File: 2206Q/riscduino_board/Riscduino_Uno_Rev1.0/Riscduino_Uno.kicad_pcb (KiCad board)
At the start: 2 copper layers, 70.1 x 54.4 mm, 93 parts, among them J1 USB_B_Micro, J10 Conn_01x01, J11 Conn_01x01, J2 ISP, J3 Conn_01x08_Pin, J4 Conn_01x06_Pin, J5 Conn_01x08_Pin, J6 Conn_01x10_Pin, J7 Conn_02x04_Odd_Even, J8 Conn_01x01, J9 Conn_01x01, SW1 4Pin Round Button SPST Straig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, U1 LM1117S-ADJ, U2 LM1117MP-3.3, U3 Riscduino, U4 CH340C, U5 MAX1232ESA+T, U6 W25Q32JVSS, U7 W25Q32JVSS, U8 23LC1024-I/P, X1 ASE-10.000MHZ-LC-T

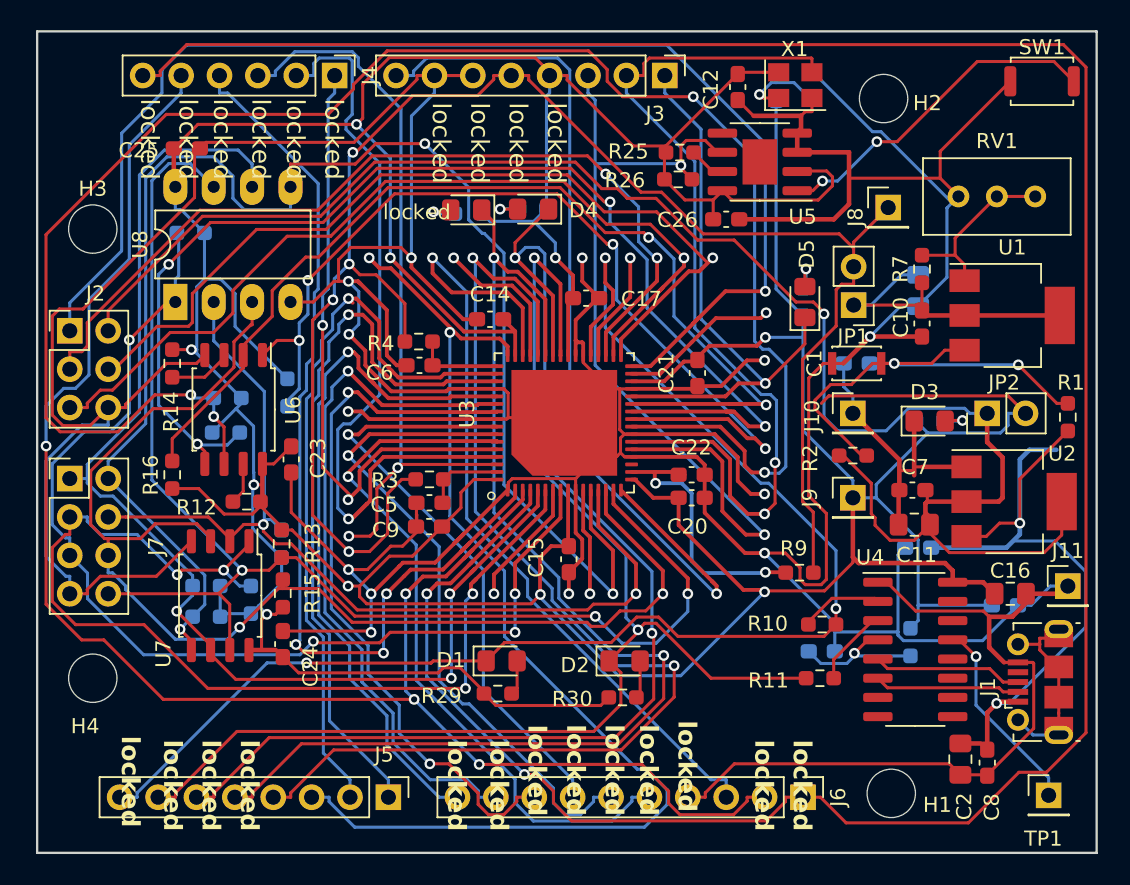
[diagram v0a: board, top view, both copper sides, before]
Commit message: 1.0.7 DRC Clean, Power Routed
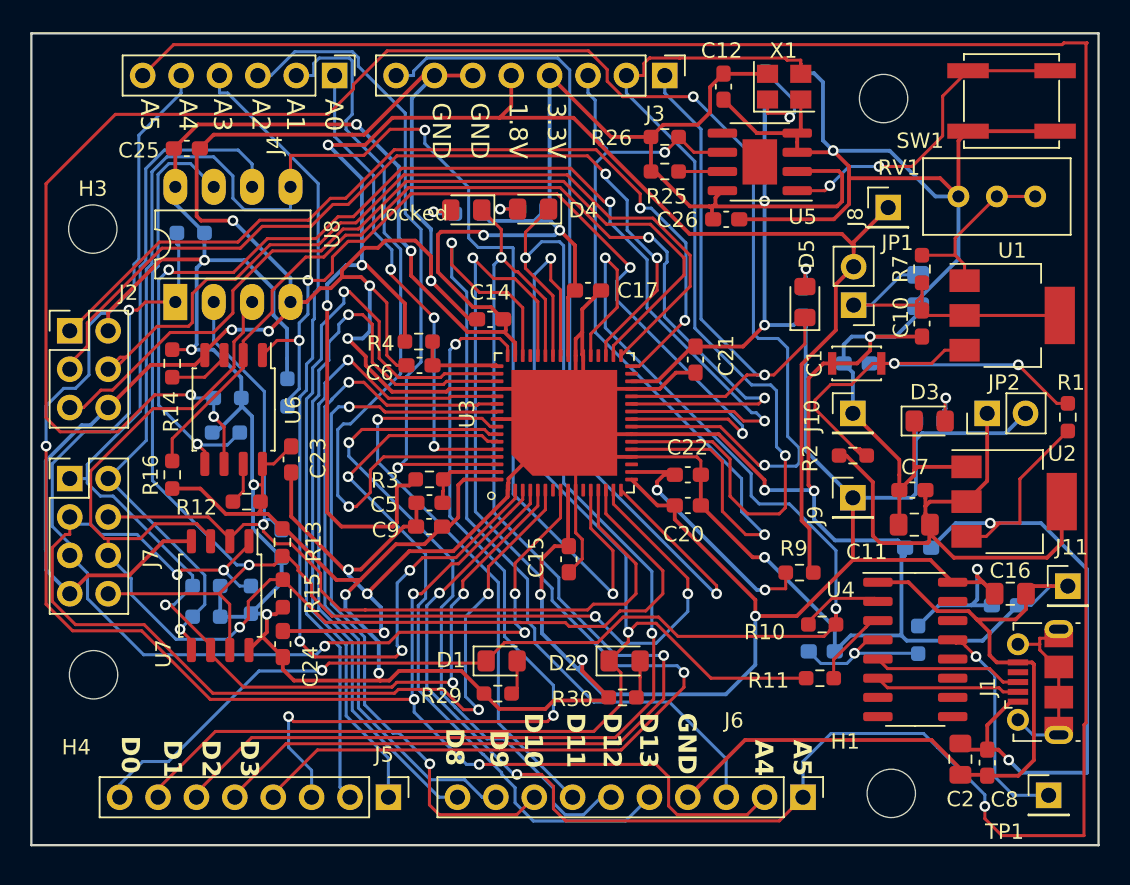
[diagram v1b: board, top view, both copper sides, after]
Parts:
- SW1: footprint Button_Switch_SMD:SW_Push_SPST_NO_Alps_SKRK -> Riscduino.Library:SW_SPST_EVPBF_TS4550TP
- U3: footprint Package_DFN_QFN:RISCDUINO_QFN-64-1EP_9x9mm_P0.5mm_EP7.65x7.65mm_NEW -> Riscduino.Library:RISCDUINO_QFN-64-1EP_9x9mm_P0.5mm_EP7.65x7.65mm_NEW
- moved R26 2.94 mm to (111.3, 56.4)
- moved SW1 2.40 mm to (134.2, 54.0), turned to 180 degrees
- moved R25 1.60 mm to (111.3, 58.7)
- moved C12 0.94 mm to (115.1, 53.1)
- moved C21 0.90 mm to (113.3, 71.1)
- moved X1 0.74 mm to (119.2, 53.1)
- moved R6 0.74 mm to (120.2, 53.1)
- moved R5 0.72 mm to (117.9, 53.0)
- moved C20 0.57 mm to (112.8, 80.8)
- moved R8 0.53 mm to (128.0, 89.7)
- moved C17 0.52 mm to (106.2, 66.5)
- moved C22 0.25 mm to (112.8, 78.7)
- moved H4 0.23 mm to (73.5, 92.0)
- moved R13 0.11 mm to (86.0, 83.2)
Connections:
- J2 pad 2: +3.3VP -> +3.3V
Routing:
- net +3.3VP: track 112.5 -> 36.0 mm, vias 1 -> 0
- net ISP_MISO: track 84.4 -> 58.1 mm, vias 1 -> 2
- net ardunio_d5: track 75.2 -> 55.8 mm, vias 2 -> 3
- net GND: track 464.5 -> 449.9 mm, vias 13 -> 14
- net ardunio_a5: track 176.4 -> 187.4 mm, vias 2 -> 3
- net mprj_io_0: track 10.6 -> 0.00 mm, vias 1 -> 0
- net mprj_io_11: track 9.76 -> 0.00 mm, vias 1 -> 0
- net ardunio_a0: track 40.9 -> 31.6 mm, vias 2 -> 3
- net mprj_io_30: track 8.48 -> 0.00 mm, vias 1 -> 0
- net mprj_io_5_ser_rx: track 7.34 -> 0.00 mm, vias 1 -> 0
- net mprj_io_32: track 7.04 -> 0.00 mm, vias 1 -> 0
- net ardunio_a2: track 49.5 -> 43.6 mm, vias 2 -> 1
- net CARAVEL_FLASH_SSN: track 63.0 -> 60.2 mm
- net CARAVEL_FLASH_SCK: track 118.6 -> 121.2 mm
- net +3.3V: track 394.8 -> 397.3 mm, vias 10 -> 16
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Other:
- board size 70.1 x 54.4 mm -> 70.6 x 53.7 mm
- board text added: "1.8V"
- board text added: "3.3V"
- board text added: "A0"
- board text added: "A1"
- board text added: "A2"
- board text added: "A3"
- board text added: "A4"
- board text added: "A5"
- board text added: "D0"
- board text added: "D1"
- board text added: "D10"
- board text added: "D11"
- board text added: "D12"
- board text added: "D13"
- board text added: "D2"
- board text added: "D3"
- board text added: "D8"
- board text added: "D9"
- board text added: "GND"
- board text added: "Riscduino Uno Rev 1.0 July 2023"
- board text removed: "locked"
